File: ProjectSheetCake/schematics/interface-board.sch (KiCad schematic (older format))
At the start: 46 parts, among them P1 CONN_8, P2 CONN_6, P3 CONN_8, P4 CONN_6, P7 X_Y_SERVO, P8 Z_A_SERVO

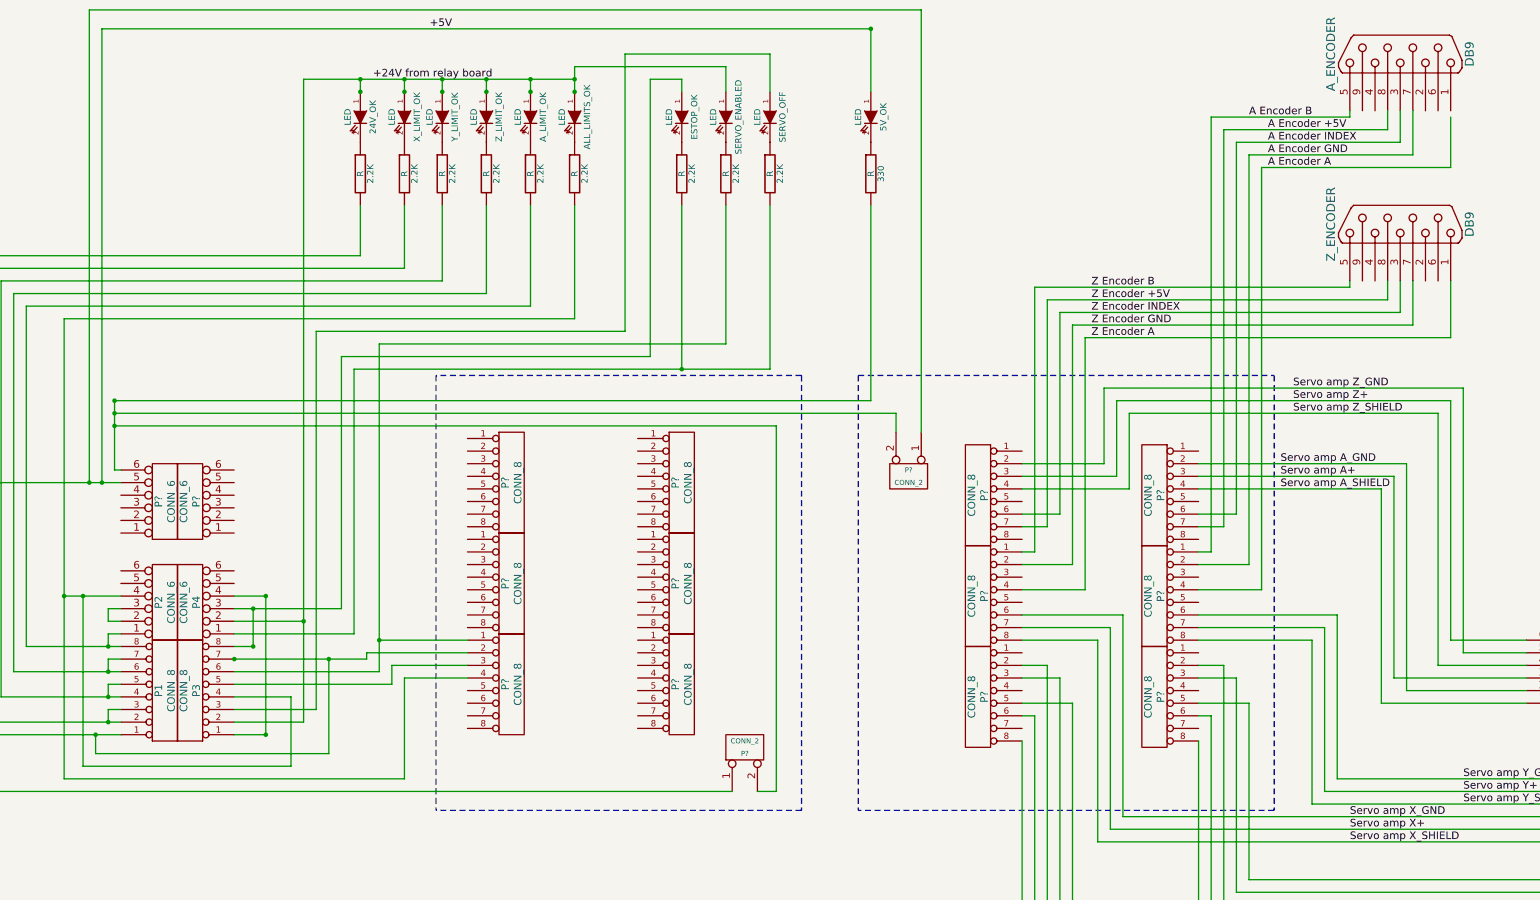
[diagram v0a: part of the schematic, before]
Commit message: fix up board layout
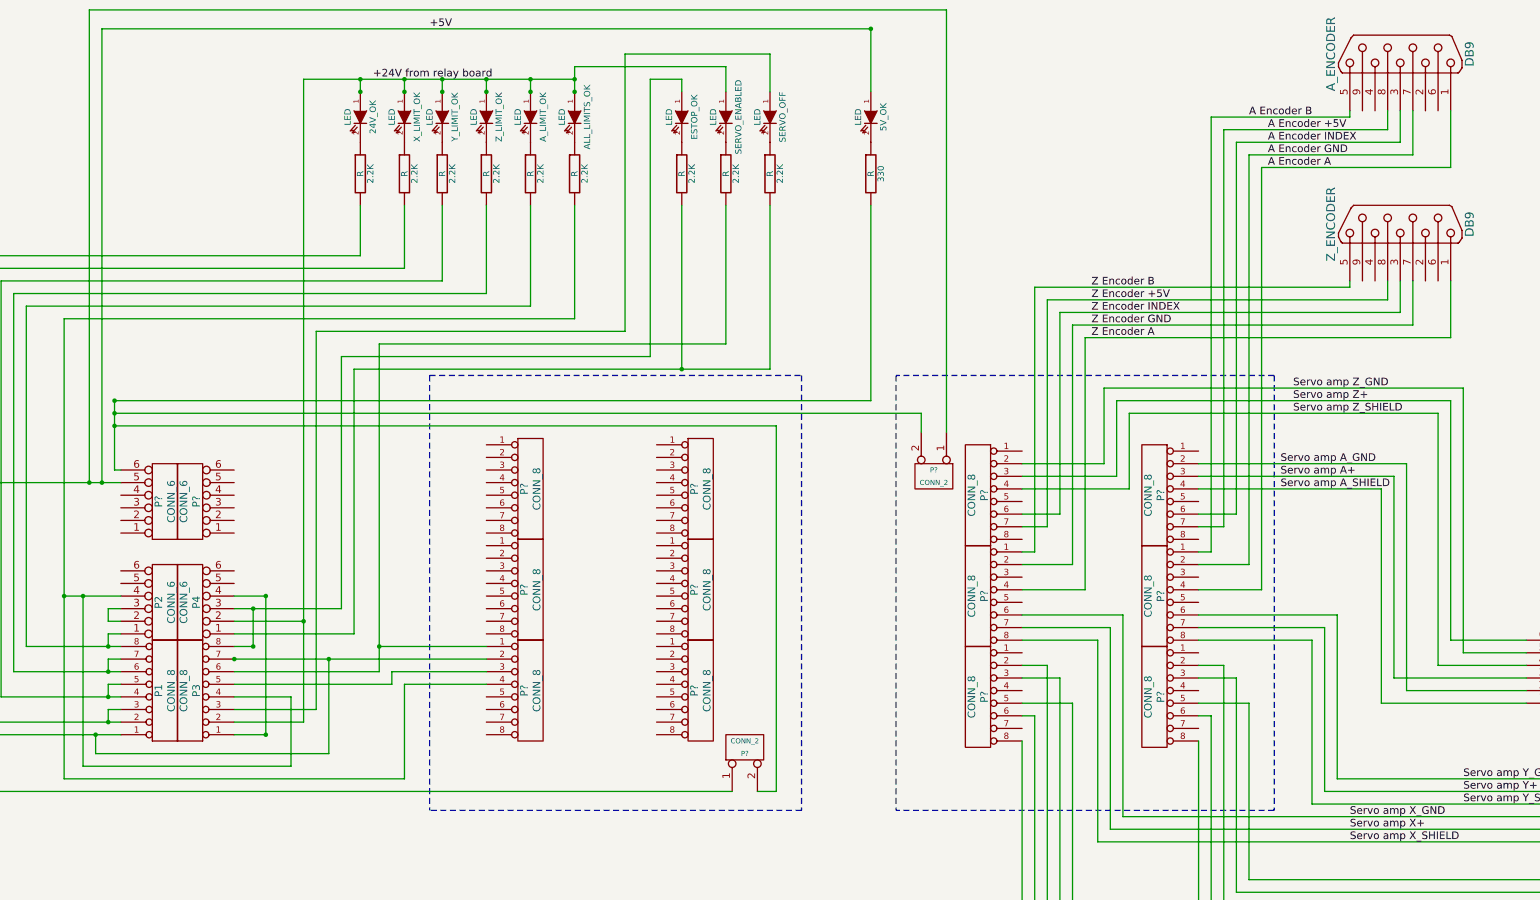
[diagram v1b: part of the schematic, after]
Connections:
- wire segments 261 -> 259
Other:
- moved on the sheet: P?
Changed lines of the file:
@@
-EESchema Schematic File Version 2  date 8/15/2011 12:07:04 AM
+EESchema Schematic File Version 2  date 8/15/2011 11:11:12 PM
 LIBS:power
 LIBS:device
@@
 Sheet 1 1
 Title ""
-Date "15 aug 2011"
+Date "16 aug 2011"
 Rev ""
 Comp ""
@@
 $EndDescr
 Wire Notes Line
-	4450 3600 4450 7050
+	11100 7050 8100 7050
 Wire Notes Line
-	7350 3600 4450 3600
+	11100 3600 8100 3600
+Wire Wire Line
+	8500 700  1700 700
+Wire Notes Line
+	4400 3600 7350 3600
+Wire Notes Line
+	4400 3600 4400 7050
+Wire Wire Line
+	4850 5950 4100 5950
+Connection ~ 4000 5750
+Wire Wire Line
+	4000 5750 4850 5750
+Wire Wire Line
+	2850 5850 4850 5850
 Wire Notes Line
 	7350 3600 7350 7050
-Wire Notes Line
-	7800 3600 7800 7050
-Wire Notes Line
-	7800 3600 11100 3600
 Wire Wire Line
 	6750 3350 4000 3350
@@
 	600  6900 6800 6900
 Wire Wire Line
-	8100 4050 8100 3900
+	8300 4050 8300 3900
 Wire Wire Line
 	1900 3800 1900 4350
@@
 Connection ~ 1900 3800
 Wire Wire Line
-	8100 3900 1900 3900
-Wire Wire Line
 	1900 4350 1950 4350
 Wire Wire Line
 	3600 6600 1750 6600
-Wire Wire Line
-	2850 5850 3900 5850
 Connection ~ 2850 5850
 Wire Wire Line
@@
 	11000 1950 12500 1950
 Wire Wire Line
-	12500 1950 12500 1550
-Wire Wire Line
 	10500 5000 10600 5000
 Wire Wire Line
@@
 	3850 1350 3850 1250
 Wire Wire Line
-	4000 5700 4700 5700
-Wire Wire Line
 	2850 5950 4000 5950
 Wire Wire Line
 	1750 6600 1750 6450
 Wire Wire Line
-	4100 5900 4100 6050
-Wire Wire Line
 	1950 5350 1500 5350
 Wire Wire Line
 	1500 6800 4200 6800
 Wire Wire Line
-	4200 6800 4200 6000
-Wire Wire Line
-	4200 6000 4700 6000
-Wire Wire Line
 	2849 6450 3099 6450
 Wire Wire Line
@@
 	3400 1250 5550 1250
 Wire Wire Line
-	4100 5900 4700 5900
-Wire Wire Line
-	4100 6050 2850 6050
+	2850 6050 4100 6050
 Wire Wire Line
 	2850 6150 3300 6150
@@
 	1650 6700 1650 5350
 Connection ~ 1650 5350
-Wire Wire Line
-	3900 5850 3900 5800
-Wire Wire Line
-	3900 5800 4700 5800
 Connection ~ 3000 5750
 Connection ~ 3000 5450
@@
 	7150 4000 7150 6900
 Wire Wire Line
-	8300 4050 8300 700
-Wire Wire Line
-	8300 700  1700 700
+	8500 700  8500 4050
 Wire Wire Line
 	1700 700  1700 4450
@@
 Wire Wire Line
 	4000 5950 4000 3350
-Connection ~ 4000 5700
-Wire Notes Line
-	7350 7050 4450 7050
 Wire Notes Line
 	11100 3600 11100 7050
+Wire Wire Line
+	12500 1950 12500 1500
+Wire Wire Line
+	4850 6050 4200 6050
+Wire Wire Line
+	4200 6050 4200 6800
+Wire Wire Line
+	4100 6050 4100 5950
 Wire Notes Line
-	11100 7050 7800 7050
+	7350 7050 4400 7050
+Wire Wire Line
+	8300 3900 1900 3900
+Wire Notes Line
+	8100 3600 8100 7050
 $Comp
 L CONN_2 P?
@@
 L CONN_2 P?
 U 1 1 4E4601E7
-P 8200 4400
-F 0 "P?" V 8150 4400 40  0000 C CNN
-F 1 "CONN_2" V 8250 4400 40  0000 C CNN
-	1    8200 4400
+P 8400 4400
+F 0 "P?" V 8350 4400 40  0000 C CNN
+F 1 "CONN_2" V 8450 4400 40  0000 C CNN
+	1    8400 4400
 	0    1    1    0
 $EndComp
@@
 L CONN_8 P?
 U 1 1 4E3F5325
-P 6400 6050
-F 0 "P?" V 6350 6050 60  0000 C CNN
-F 1 "CONN_8" V 6450 6050 60  0000 C CNN
-	1    6400 6050
+P 6550 6100
+F 0 "P?" V 6500 6100 60  0000 C CNN
+F 1 "CONN_8" V 6600 6100 60  0000 C CNN
+	1    6550 6100
 	1    0    0    -1
 $EndComp
@@
 L CONN_8 P?
 U 1 1 4E3F5321
-P 6400 5250
-F 0 "P?" V 6350 5250 60  0000 C CNN
-F 1 "CONN_8" V 6450 5250 60  0000 C CNN
-	1    6400 5250
+P 6550 5300
+F 0 "P?" V 6500 5300 60  0000 C CNN
+F 1 "CONN_8" V 6600 5300 60  0000 C CNN
+	1    6550 5300
 	1    0    0    -1
 $EndComp
@@
 L CONN_8 P?
 U 1 1 4E3F531C
-P 6400 4450
-F 0 "P?" V 6350 4450 60  0000 C CNN
-F 1 "CONN_8" V 6450 4450 60  0000 C CNN
-	1    6400 4450
+P 6550 4500
+F 0 "P?" V 6500 4500 60  0000 C CNN
+F 1 "CONN_8" V 6600 4500 60  0000 C CNN
+	1    6550 4500
 	1    0    0    -1
 $EndComp
@@
 L CONN_8 P?
 U 1 1 4E3F5317
-P 5050 6050
-F 0 "P?" V 5000 6050 60  0000 C CNN
-F 1 "CONN_8" V 5100 6050 60  0000 C CNN
-	1    5050 6050
+P 5200 6100
+F 0 "P?" V 5150 6100 60  0000 C CNN
+F 1 "CONN_8" V 5250 6100 60  0000 C CNN
+	1    5200 6100
 	1    0    0    -1
 $EndComp
@@
 L CONN_8 P?
 U 1 1 4E3F5313
-P 5050 5250
-F 0 "P?" V 5000 5250 60  0000 C CNN
-F 1 "CONN_8" V 5100 5250 60  0000 C CNN
-	1    5050 5250
+P 5200 5300
+F 0 "P?" V 5150 5300 60  0000 C CNN
+F 1 "CONN_8" V 5250 5300 60  0000 C CNN
+	1    5200 5300
 	1    0    0    -1
 $EndComp
@@
 L CONN_8 P?
 U 1 1 4E3F530D
-P 5050 4450
-F 0 "P?" V 5000 4450 60  0000 C CNN
-F 1 "CONN_8" V 5100 4450 60  0000 C CNN
-	1    5050 4450
-	1    0    0    -1
-$EndComp
+P 5200 4500
+F 0 "P?" V 5150 4500 60  0000 C CNN
+F 1 "CONN_8" V 5250 4500 60  0000 C CNN
+	1    5200 4500
+	1    0    0    -1
+$EndComp
